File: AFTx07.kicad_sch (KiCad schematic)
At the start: 1 part

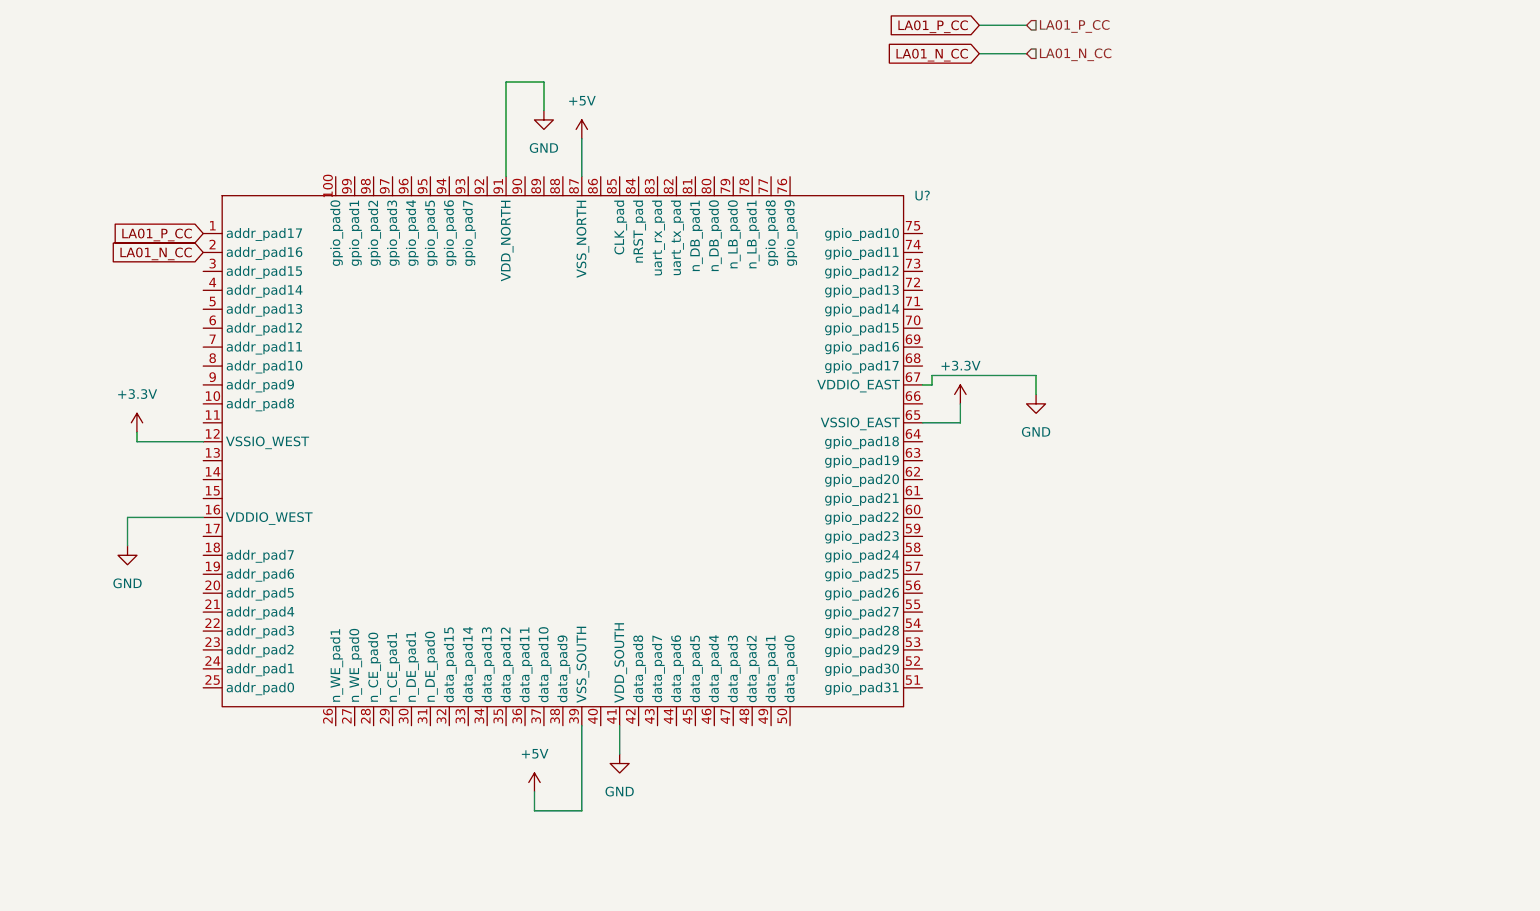
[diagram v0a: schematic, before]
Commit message: Add files via upload
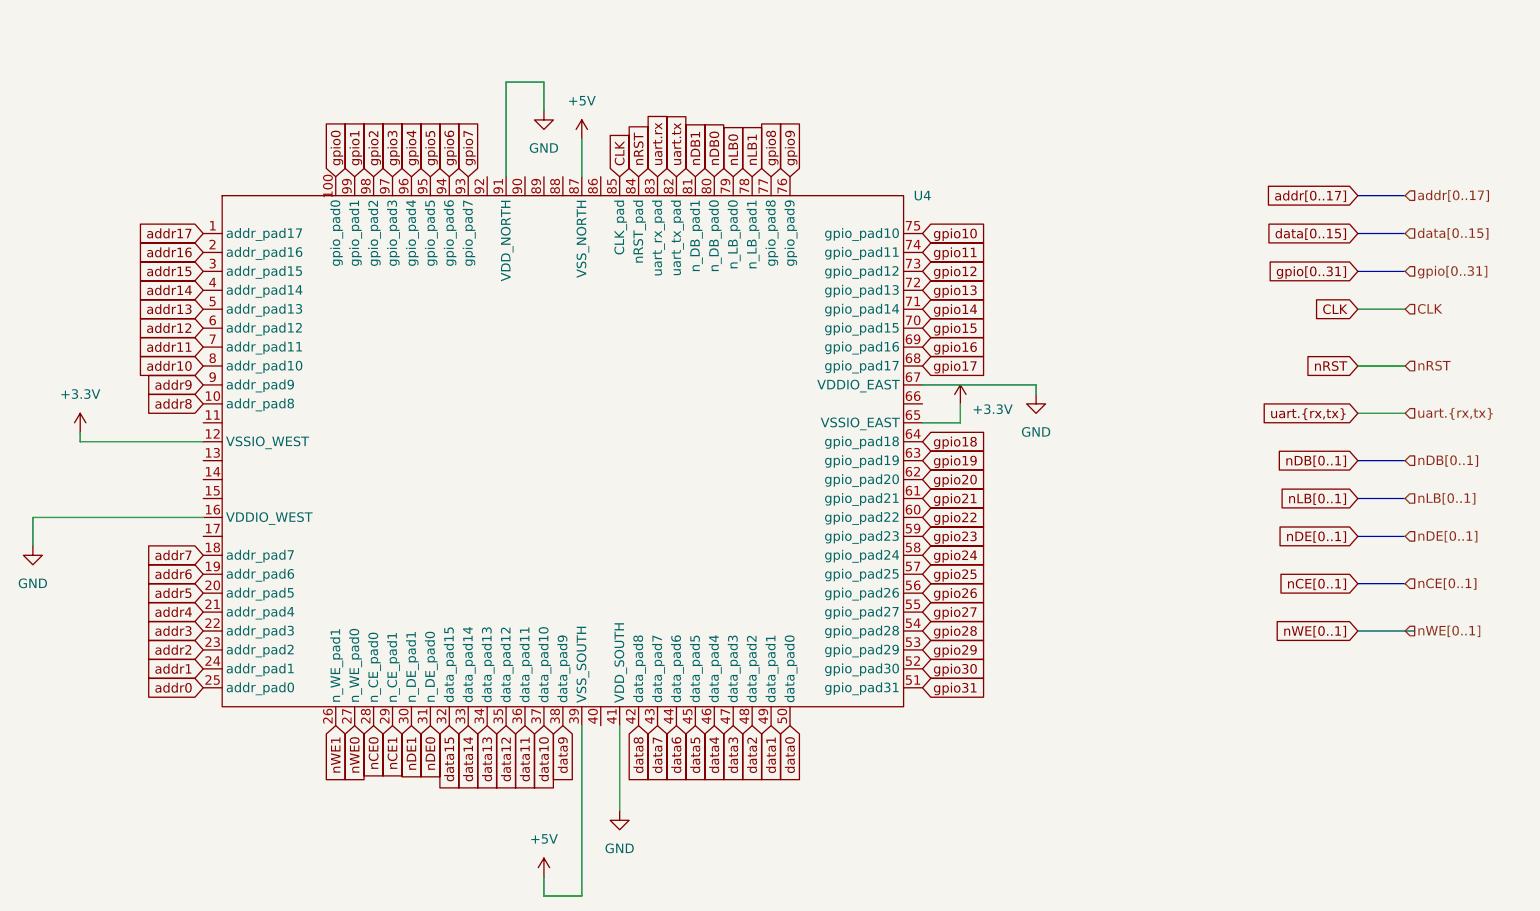
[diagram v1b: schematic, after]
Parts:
- gave numbers to parts that had none: 1
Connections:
- net addr8: now reaches U4.10 (addr_pad8)
- net gpio0: now reaches U4.100 (gpio_pad0)
- net addr7: now reaches U4.18 (addr_pad7)
- net addr6: now reaches U4.19 (addr_pad6)
- net addr5: now reaches U4.20 (addr_pad5)
- net addr4: now reaches U4.21 (addr_pad4)
- net addr3: now reaches U4.22 (addr_pad3)
- net addr2: now reaches U4.23 (addr_pad2)
- net addr1: now reaches U4.24 (addr_pad1)
- net addr0: now reaches U4.25 (addr_pad0)
- net nWE1: now reaches U4.26 (n_WE_pad1)
- net nWE0: now reaches U4.27 (n_WE_pad0)
- net nCE0: now reaches U4.28 (n_CE_pad0)
- net nCE1: now reaches U4.29 (n_CE_pad1)
- net addr15: now reaches U4.3 (addr_pad15)
- net nDE1: now reaches U4.30 (n_DE_pad1)
- net nDE0: now reaches U4.31 (n_DE_pad0)
- net data15: now reaches U4.32 (data_pad15)
- net data14: now reaches U4.33 (data_pad14)
- net data13: now reaches U4.34 (data_pad13)
- net data12: now reaches U4.35 (data_pad12)
- net data11: now reaches U4.36 (data_pad11)
- net data10: now reaches U4.37 (data_pad10)
- net data9: now reaches U4.38 (data_pad9)
- net addr14: now reaches U4.4 (addr_pad14)
- net data8: now reaches U4.42 (data_pad8)
- net data7: now reaches U4.43 (data_pad7)
- net data6: now reaches U4.44 (data_pad6)
- net data5: now reaches U4.45 (data_pad5)
- net data4: now reaches U4.46 (data_pad4)
- net data3: now reaches U4.47 (data_pad3)
- net data2: now reaches U4.48 (data_pad2)
- net data1: now reaches U4.49 (data_pad1)
- net addr13: now reaches U4.5 (addr_pad13)
- net data0: now reaches U4.50 (data_pad0)
- net gpio31: now reaches U4.51 (gpio_pad31)
- net gpio30: now reaches U4.52 (gpio_pad30)
- net gpio29: now reaches U4.53 (gpio_pad29)
- net gpio28: now reaches U4.54 (gpio_pad28)
- net gpio27: now reaches U4.55 (gpio_pad27)
- net gpio26: now reaches U4.56 (gpio_pad26)
- net gpio25: now reaches U4.57 (gpio_pad25)
- net gpio24: now reaches U4.58 (gpio_pad24)
- net gpio23: now reaches U4.59 (gpio_pad23)
- net addr12: now reaches U4.6 (addr_pad12)
- net gpio22: now reaches U4.60 (gpio_pad22)
- net gpio21: now reaches U4.61 (gpio_pad21)
- net gpio20: now reaches U4.62 (gpio_pad20)
- net gpio19: now reaches U4.63 (gpio_pad19)
- net gpio18: now reaches U4.64 (gpio_pad18)
- net gpio17: now reaches U4.68 (gpio_pad17)
- net gpio16: now reaches U4.69 (gpio_pad16)
- net addr11: now reaches U4.7 (addr_pad11)
- net gpio15: now reaches U4.70 (gpio_pad15)
- net gpio14: now reaches U4.71 (gpio_pad14)
- net gpio13: now reaches U4.72 (gpio_pad13)
- net gpio12: now reaches U4.73 (gpio_pad12)
- net gpio11: now reaches U4.74 (gpio_pad11)
- net gpio10: now reaches U4.75 (gpio_pad10)
- net gpio9: now reaches U4.76 (gpio_pad9)
- net gpio8: now reaches U4.77 (gpio_pad8)
- net nLB1: now reaches U4.78 (n_LB_pad1)
- net nLB0: now reaches U4.79 (n_LB_pad0)
- net addr10: now reaches U4.8 (addr_pad10)
- net nDB0: now reaches U4.80 (n_DB_pad0)
- net nDB1: now reaches U4.81 (n_DB_pad1)
- net uart.tx: now reaches U4.82 (uart_tx_pad)
- net uart.rx: now reaches U4.83 (uart_rx_pad)
- net nRST: now reaches U4.84 (nRST_pad)
- net CLK: now reaches U4.85 (CLK_pad)
- net addr9: now reaches U4.9 (addr_pad9)
- net gpio7: now reaches U4.93 (gpio_pad7)
- net gpio6: now reaches U4.94 (gpio_pad6)
- net gpio5: now reaches U4.95 (gpio_pad5)
- net gpio4: now reaches U4.96 (gpio_pad4)
- net gpio3: now reaches U4.97 (gpio_pad3)
- net gpio2: now reaches U4.98 (gpio_pad2)
- net gpio1: now reaches U4.99 (gpio_pad1)
- net LA01_N_CC renamed addr16
- net LA01_P_CC renamed addr17

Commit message: Add files via upload
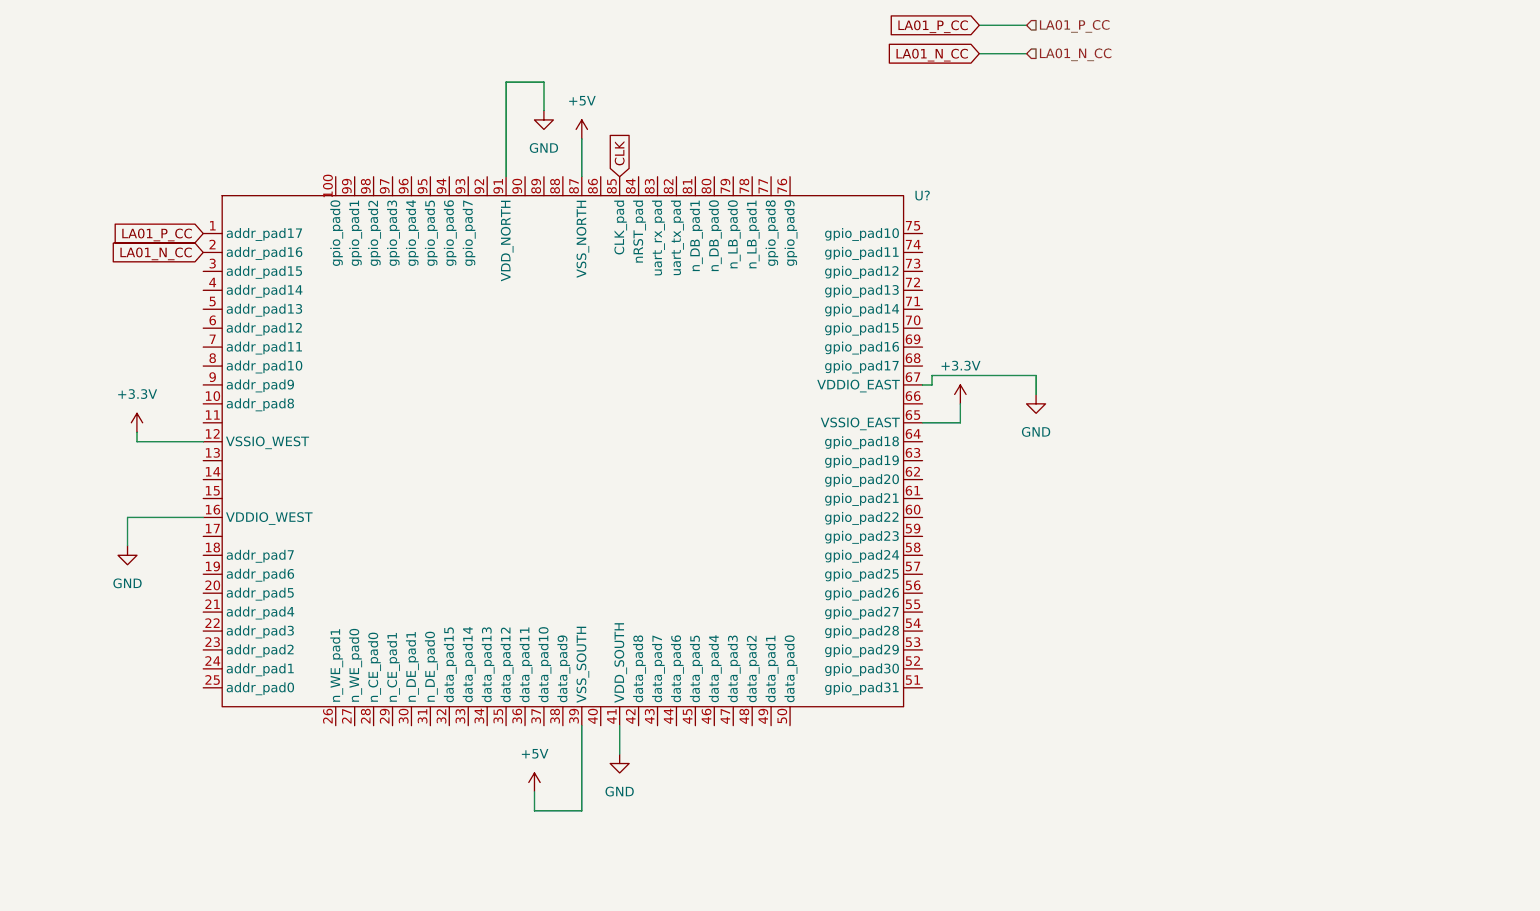
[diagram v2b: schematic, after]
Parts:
- renumbered U4 to U?
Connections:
- net addr0: no longer names the net of U?.25 (addr_pad0)
- net addr1: no longer names the net of U?.24 (addr_pad1)
- net addr10: no longer names the net of U?.8 (addr_pad10)
- net addr11: no longer names the net of U?.7 (addr_pad11)
- net addr12: no longer names the net of U?.6 (addr_pad12)
- net addr13: no longer names the net of U?.5 (addr_pad13)
- net addr14: no longer names the net of U?.4 (addr_pad14)
- net addr15: no longer names the net of U?.3 (addr_pad15)
- net addr16 renamed LA01_N_CC
- net addr17 renamed LA01_P_CC
- net addr2: no longer names the net of U?.23 (addr_pad2)
- net addr3: no longer names the net of U?.22 (addr_pad3)
- net addr4: no longer names the net of U?.21 (addr_pad4)
- net addr5: no longer names the net of U?.20 (addr_pad5)
- net addr6: no longer names the net of U?.19 (addr_pad6)
- net addr7: no longer names the net of U?.18 (addr_pad7)
- net addr8: no longer names the net of U?.10 (addr_pad8)
- net addr9: no longer names the net of U?.9 (addr_pad9)
- net data0: no longer names the net of U?.50 (data_pad0)
- net data1: no longer names the net of U?.49 (data_pad1)
- net data10: no longer names the net of U?.37 (data_pad10)
- net data11: no longer names the net of U?.36 (data_pad11)
- net data12: no longer names the net of U?.35 (data_pad12)
- net data13: no longer names the net of U?.34 (data_pad13)
- net data14: no longer names the net of U?.33 (data_pad14)
- net data15: no longer names the net of U?.32 (data_pad15)
- net data2: no longer names the net of U?.48 (data_pad2)
- net data3: no longer names the net of U?.47 (data_pad3)
- net data4: no longer names the net of U?.46 (data_pad4)
- net data5: no longer names the net of U?.45 (data_pad5)
- net data6: no longer names the net of U?.44 (data_pad6)
- net data7: no longer names the net of U?.43 (data_pad7)
- net data8: no longer names the net of U?.42 (data_pad8)
- net data9: no longer names the net of U?.38 (data_pad9)
- net gpio0: no longer names the net of U?.100 (gpio_pad0)
- net gpio1: no longer names the net of U?.99 (gpio_pad1)
- net gpio10: no longer names the net of U?.75 (gpio_pad10)
- net gpio11: no longer names the net of U?.74 (gpio_pad11)
- net gpio12: no longer names the net of U?.73 (gpio_pad12)
- net gpio13: no longer names the net of U?.72 (gpio_pad13)
- net gpio14: no longer names the net of U?.71 (gpio_pad14)
- net gpio15: no longer names the net of U?.70 (gpio_pad15)
- net gpio16: no longer names the net of U?.69 (gpio_pad16)
- net gpio17: no longer names the net of U?.68 (gpio_pad17)
- net gpio18: no longer names the net of U?.64 (gpio_pad18)
- net gpio19: no longer names the net of U?.63 (gpio_pad19)
- net gpio2: no longer names the net of U?.98 (gpio_pad2)
- net gpio20: no longer names the net of U?.62 (gpio_pad20)
- net gpio21: no longer names the net of U?.61 (gpio_pad21)
- net gpio22: no longer names the net of U?.60 (gpio_pad22)
- net gpio23: no longer names the net of U?.59 (gpio_pad23)
- net gpio24: no longer names the net of U?.58 (gpio_pad24)
- net gpio25: no longer names the net of U?.57 (gpio_pad25)
- net gpio26: no longer names the net of U?.56 (gpio_pad26)
- net gpio27: no longer names the net of U?.55 (gpio_pad27)
- net gpio28: no longer names the net of U?.54 (gpio_pad28)
- net gpio29: no longer names the net of U?.53 (gpio_pad29)
- net gpio3: no longer names the net of U?.97 (gpio_pad3)
- net gpio30: no longer names the net of U?.52 (gpio_pad30)
- net gpio31: no longer names the net of U?.51 (gpio_pad31)
- net gpio4: no longer names the net of U?.96 (gpio_pad4)
- net gpio5: no longer names the net of U?.95 (gpio_pad5)
- net gpio6: no longer names the net of U?.94 (gpio_pad6)
- net gpio7: no longer names the net of U?.93 (gpio_pad7)
- net gpio8: no longer names the net of U?.77 (gpio_pad8)
- net gpio9: no longer names the net of U?.76 (gpio_pad9)
- net nCE0: no longer names the net of U?.28 (n_CE_pad0)
- net nCE1: no longer names the net of U?.29 (n_CE_pad1)
- net nDB0: no longer names the net of U?.80 (n_DB_pad0)
- net nDB1: no longer names the net of U?.81 (n_DB_pad1)
- net nDE0: no longer names the net of U?.31 (n_DE_pad0)
- net nDE1: no longer names the net of U?.30 (n_DE_pad1)
- net nLB0: no longer names the net of U?.79 (n_LB_pad0)
- net nLB1: no longer names the net of U?.78 (n_LB_pad1)
- net nRST: no longer names the net of U?.84 (nRST_pad)
- net nWE0: no longer names the net of U?.27 (n_WE_pad0)
- net nWE1: no longer names the net of U?.26 (n_WE_pad1)
- net uart.rx: no longer names the net of U?.83 (uart_rx_pad)
- net uart.tx: no longer names the net of U?.82 (uart_tx_pad)
